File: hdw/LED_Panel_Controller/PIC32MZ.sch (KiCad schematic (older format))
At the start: 3 parts, among them U1101 PIC32MZ2048EFG100_IPF

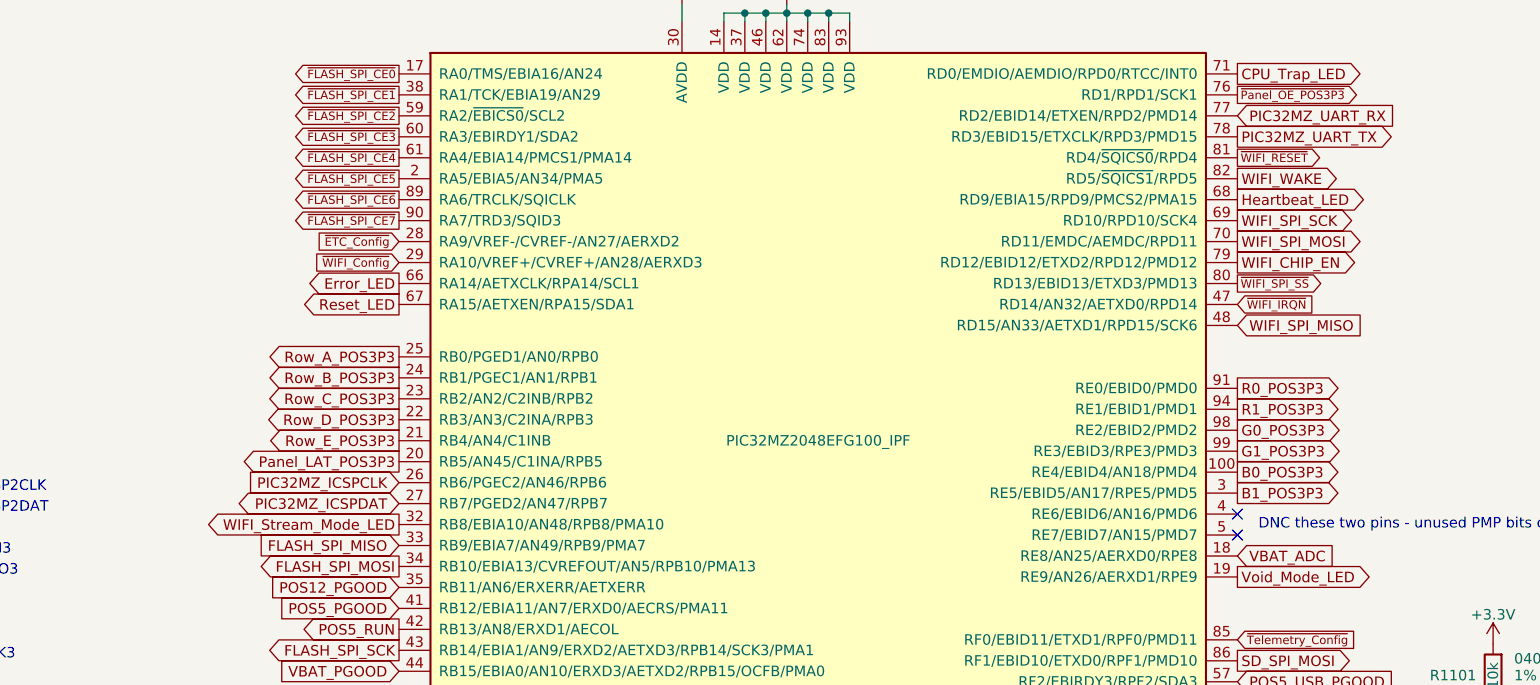
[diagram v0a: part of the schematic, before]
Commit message: having a mid-project crisis
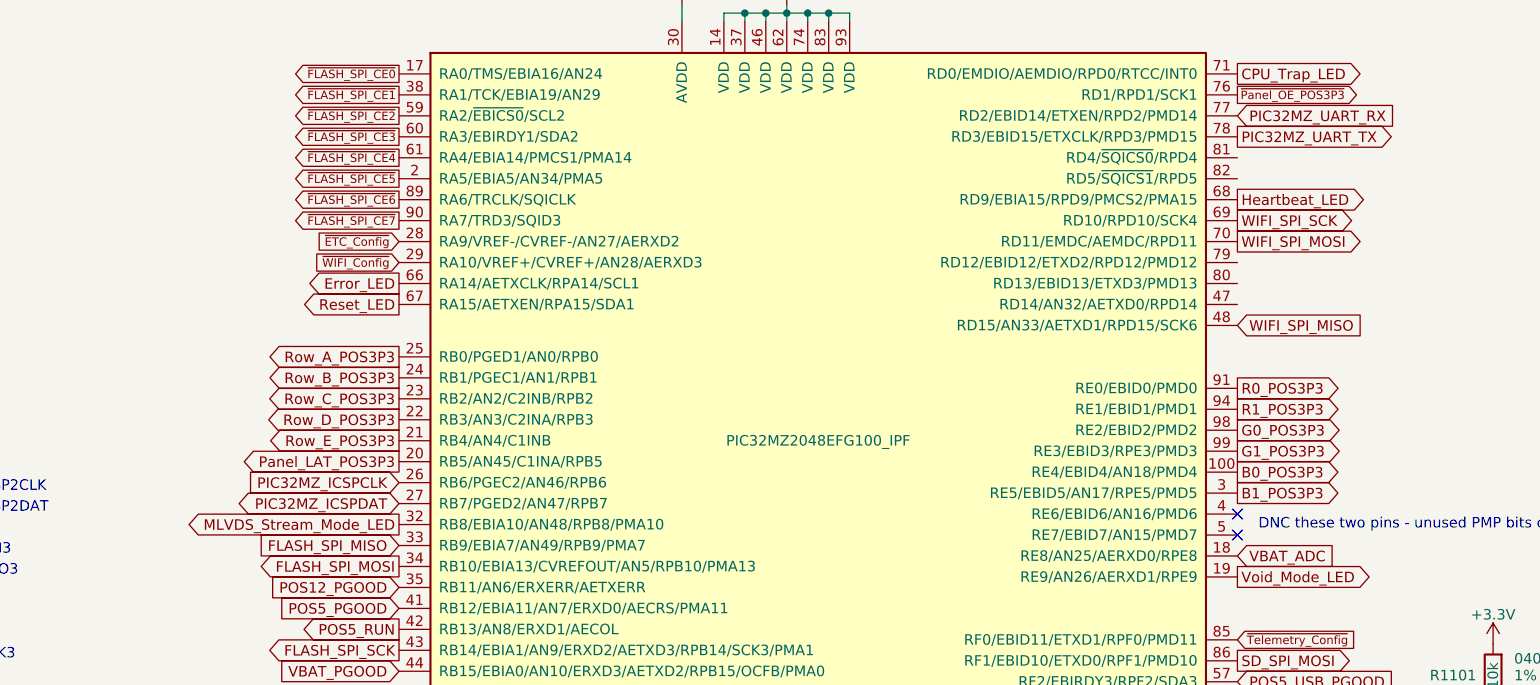
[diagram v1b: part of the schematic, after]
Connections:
- net WIFI_CHIP_EN: no longer names the net of U1101.79 (RD12/EBID12/ETXD2/RPD12/PMD12)
- net WIFI_Stream_Mode_LED renamed MLVDS_Stream_Mode_LED
- net WIFI_WAKE: no longer names the net of U1101.82 (RD5/~SQICS1~/RPD5)
- net ~WIFI_IRQN: no longer names the net of U1101.47 (RD14/AN32/AETXD0/RPD14)
- net ~WIFI_RESET: no longer names the net of U1101.81 (RD4/~SQICS0~/RPD4)
- net ~WIFI_SPI_SS: no longer names the net of U1101.80 (RD13/EBID13/ETXD3/PMD13)
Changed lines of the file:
@@
 Text GLabel 3020 5000 0    50   Input ~ 0
 PIC32MZ_SOSC_EC
-Text GLabel 7020 1700 2    40   Output ~ 0
-~WIFI_RESET
-Text GLabel 7020 1800 2    50   Output ~ 0
-WIFI_WAKE
-Text GLabel 7020 2200 2    50   Output ~ 0
-WIFI_CHIP_EN
 Text GLabel 7020 2000 2    50   Output ~ 0
 WIFI_SPI_SCK
-Text GLabel 7020 2300 2    40   Output ~ 0
-~WIFI_SPI_SS
 Text GLabel 7020 2100 2    50   Output ~ 0
 WIFI_SPI_MOSI
 Text GLabel 7020 2500 2    50   Input ~ 0
 WIFI_SPI_MISO
-Text GLabel 7020 2400 2    40   Input ~ 0
-~WIFI_IRQN
 $Comp
 L Custom_Library:GNDA_MZ #PWR01103
@@
 ~FLASH_SPI_CE7
 Text GLabel 3020 3450 0    50   Output ~ 0
-WIFI_Stream_Mode_LED
+MLVDS_Stream_Mode_LED
 Text Notes 9720 1950 0    50   ~ 0
 OC5
